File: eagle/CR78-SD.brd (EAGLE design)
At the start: 100 x 80 mm, 46 parts, among them Q1 2N3904, Q2 2N3904, Q3 2N3904, Q4 2N3904, Q7 2N3904

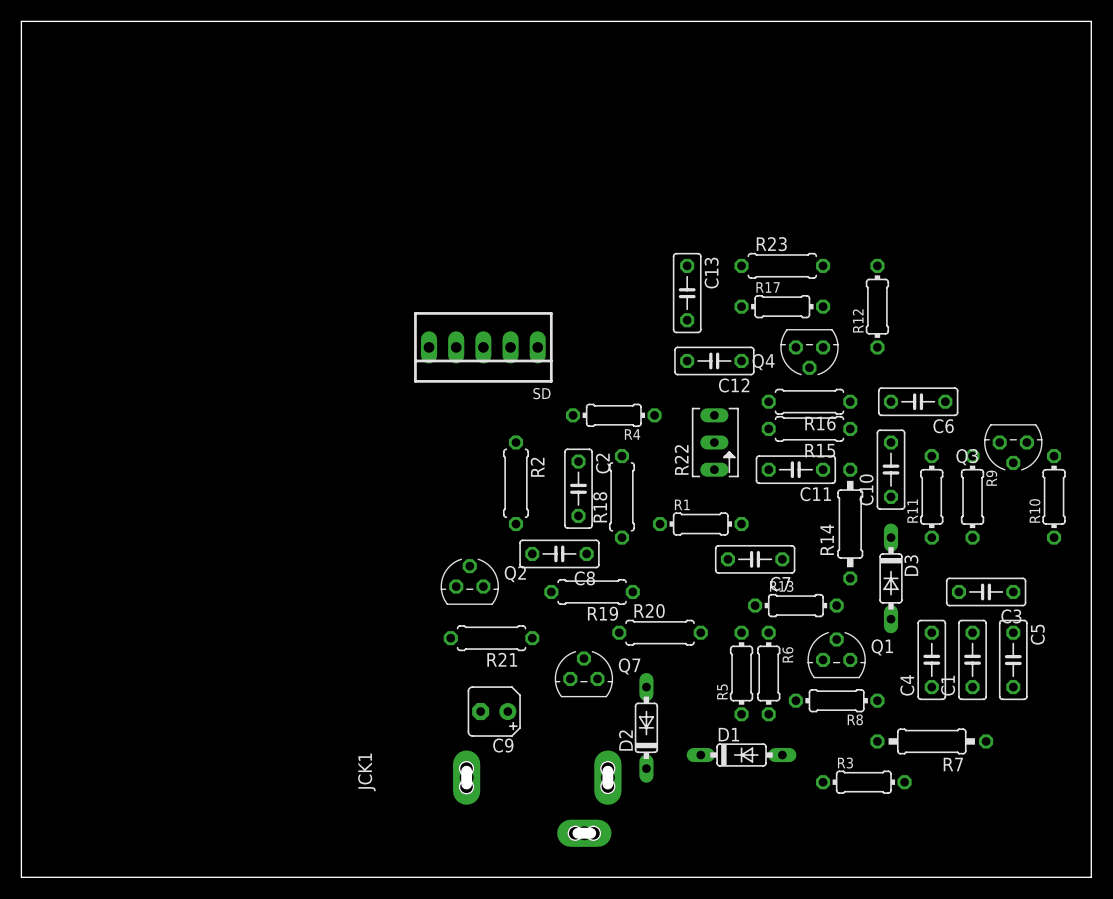
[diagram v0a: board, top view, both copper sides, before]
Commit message: 95pct auto
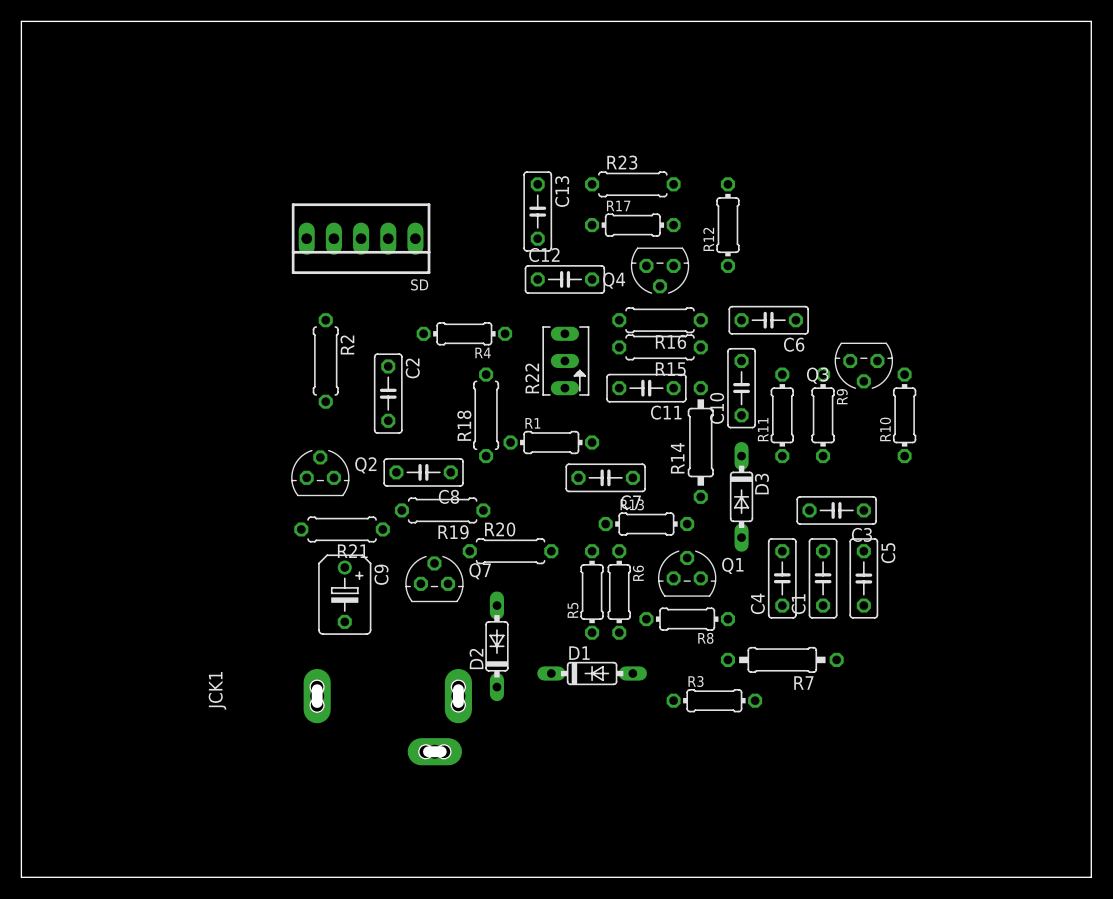
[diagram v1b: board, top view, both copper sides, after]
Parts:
- C9: device rcl:B45181A -> rcl:B45181B
- moved R2 21.1 mm to (28.4, 48.3)
- moved C2 19.9 mm to (34.3, 45.2)
- moved C9 17.7 mm to (30.2, 26.4), turned to 270 degrees
- moved Q2 17.3 mm to (27.9, 37.3)
- moved R21 17.3 mm to (30.0, 32.5)
- moved Q7 16.6 mm to (38.6, 27.4)
- moved Q1 15.9 mm to (62.2, 27.9)
- moved R17 15.9 mm to (57.1, 61.0)
- moved R19 15.9 mm to (39.4, 34.3)
- moved R23 15.9 mm to (57.1, 64.8)
- moved R8 15.9 mm to (62.2, 24.1)
- moved C12 15.9 mm to (50.8, 55.9), turned to 0 degrees
- moved R13 15.9 mm to (58.4, 33.0)
- moved R15 15.9 mm to (59.7, 49.5)
- moved C1 15.9 mm to (74.9, 27.9)
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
